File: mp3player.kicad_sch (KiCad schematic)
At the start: 3 parts, among them J1 AudioJack3, U1 ES8388, U2 ESP32-S3-WROOM-1

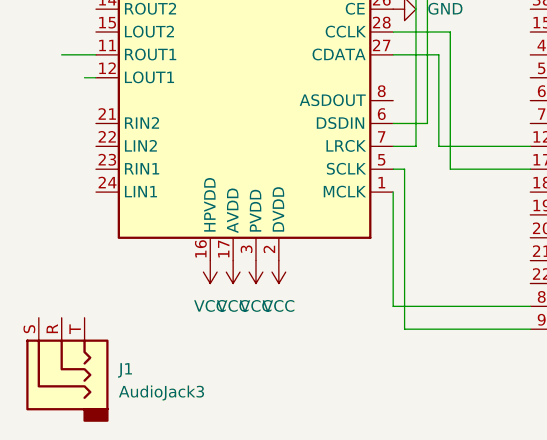
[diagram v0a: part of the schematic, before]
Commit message: Autosave
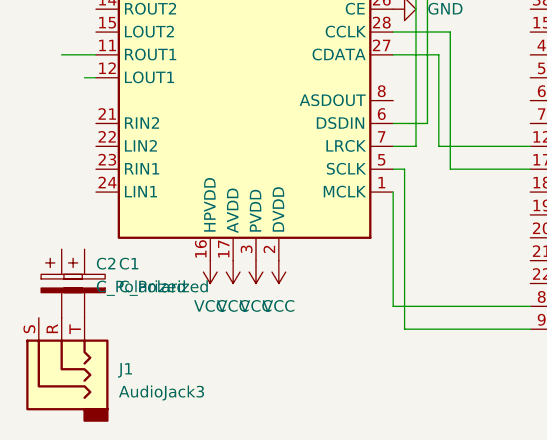
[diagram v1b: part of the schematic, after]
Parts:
- added C1, C2: C_Polarized, symbol Device:C_Polarized
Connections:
- net at J1.R: now also C2.2
- net at J1.T: now also C1.2
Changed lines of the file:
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@@
+	)
+	(symbol
+		(lib_id "Device:C_Polarized")
+		(at 17.78 64.77 0)
+		(unit 1)
+		(body_style 1)
+		(exclude_from_sim no)
+		(in_bom yes)
+		(on_board yes)
+		(in_pos_files yes)
+		(dnp no)
+		(fields_autoplaced yes)
+		(property "Reference" "C2"
+			(at 21.59 62.6109 0)
+			(show_name no)
+			(do_not_autoplace no)
+			(effects
+				(font
+					(size 1.27 1.27)
+				)
+				(justify left)
+			)
+		)
+		(property "Value" "C_Polarized"
+			(at 21.59 65.1509 0)
+			(show_name no)
+			(do_not_autoplace no)
+			(effects
+				(font
+					(size 1.27 1.27)
+				)
+				(justify left)
+			)
+		)
+		(property "Footprint" ""
+			(at 18.7452 68.58 0)
+			(hide yes)
+			(show_name no)
+			(do_not_autoplace no)
+			(effects
+				(font
+					(size 1.27 1.27)
+				)
+			)
+		)
+		(property "Datasheet" ""
+			(at 17.78 64.77 0)
+			(hide yes)
+			(show_name no)
+			(do_not_autoplace no)
+			(effects
+				(font
+					(size 1.27 1.27)
+				)
+			)
+		)
+		(property "Description" "Polarized capacitor"
+			(at 17.78 64.77 0)
+			(hide yes)
+			(show_name no)
+			(do_not_autoplace no)
+			(effects
+				(font
+					(size 1.27 1.27)
+				)
+			)
+		)
+		(pin "1"
+		)
+		(pin "2"
+		)
+		(instances
+			(project "mp3player"
+				(path "/7851373b-cb7e-4e42-801a-d8b5ac5735f4"
+					(reference "C2")
+					(unit 1)
+				)
+			)
+		)
 	)
 	(symbol
@@
 					(unit 1)
 				)
+			)
+		)
+	)
+	(symbol
+		(lib_id "Device:C_Polarized")
+		(at 20.32 64.77 0)
+		(unit 1)
+		(body_style 1)
+		(exclude_from_sim no)
+		(in_bom yes)
+		(on_board yes)
+		(in_pos_files yes)
+		(dnp no)
+		(fields_autoplaced yes)
+		(property "Reference" "C1"
+			(at 24.13 62.6109 0)
+			(show_name no)
+			(do_not_autoplace no)
+			(effects
+				(font
+					(size 1.27 1.27)
+				)
+				(justify left)
+			)
+		)
+		(property "Value" "C_Polarized"
+			(at 24.13 65.1509 0)
+			(show_name no)
+			(do_not_autoplace no)
+			(effects
+				(font
+					(size 1.27 1.27)
+				)
+				(justify left)
+			)
+		)
+		(property "Footprint" ""
+			(at 21.2852 68.58 0)
+			(hide yes)
+			(show_name no)
+			(do_not_autoplace no)
+			(effects
+				(font
+					(size 1.27 1.27)
+				)
+			)
+		)
+		(property "Datasheet" ""
+			(at 20.32 64.77 0)
+			(hide yes)
+			(show_name no)
+			(do_not_autoplace no)
+			(effects
+				(font
+					(size 1.27 1.27)
+				)
+			)
+		)
+		(property "Description" "Polarized capacitor"
+			(at 20.32 64.77 0)
+			(hide yes)
+			(show_name no)
+			(do_not_autoplace no)
+			(effects
+				(font
+					(size 1.27 1.27)
+				)
+			)
+		)
+		(pin "1"
+		)
+		(pin "2"
+		)
+		(instances
+			(project "mp3player"
+				(path "/7851373b-cb7e-4e42-801a-d8b5ac5735f4"
+					(reference "C1")
+					(unit 1)
+				)
